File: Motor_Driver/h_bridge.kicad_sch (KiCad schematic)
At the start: 52 parts, among them M1 Motor_DC, M2 Motor_DC, Q10 PMOS, Q11 CSD18540Q5B, Q12 SQJ407EP, Q13 CSD18540Q5B, Q14 MMBT3904, Q3 CSD18540Q5B, Q4 CSD18540Q5B, Q5 SQJ407EP, Q6 PMOS, Q7 MMBT3904, Q8 MMBT3904, Q9 MMBT3904, U4 UCC27524D, U5 UCC27524D

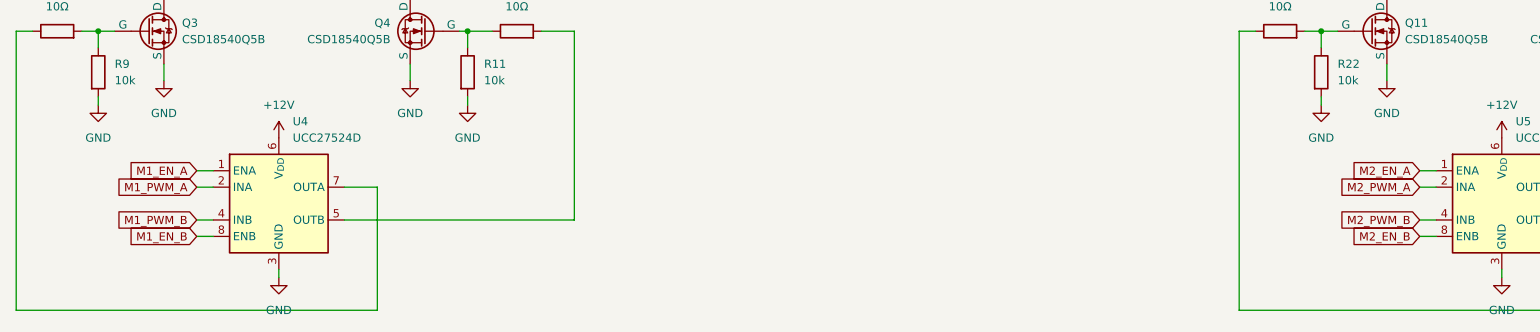
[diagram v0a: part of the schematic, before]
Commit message: Potential Finished Schematic Before Placements
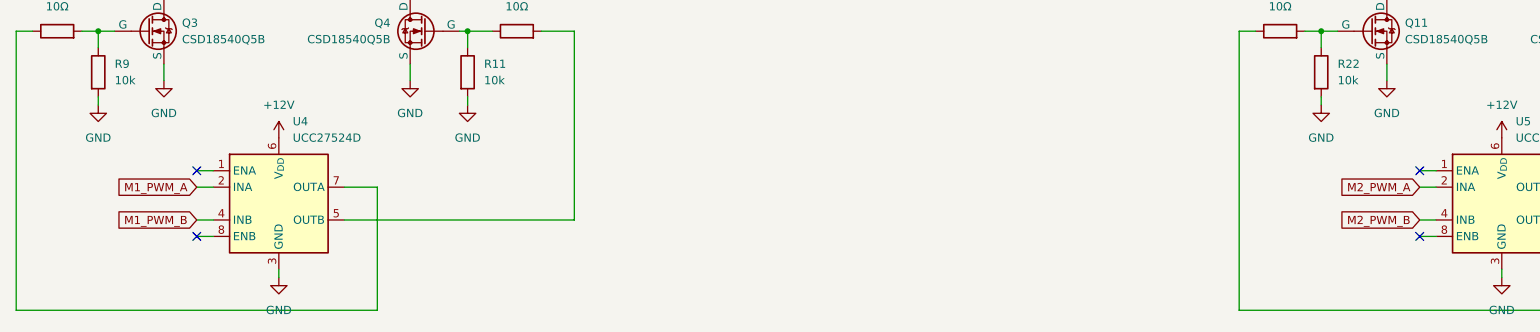
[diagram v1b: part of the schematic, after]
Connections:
- net M1_EN_A: no longer names the net of U4.1 (ENA)
- net M1_EN_B: no longer names the net of U4.8 (ENB)
- net M2_EN_A: no longer names the net of U5.1 (ENA)
- net M2_EN_B: no longer names the net of U5.8 (ENB)
- no-connect marks 0 -> 4
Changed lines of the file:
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@@
 		(color 0 0 0 0)
+	)
+	(no_connect
+		(at 292.1 190.5)
+	)
+	(no_connect
+		(at 102.87 190.5)
+	)
+	(no_connect
+		(at 292.1 180.34)
+	)
+	(no_connect
+		(at 102.87 180.34)
 	)
 	(wire
@@
 		)
 	)
-	(global_label "M2_EN_B"
-		(shape input)
-		(at 292.1 190.5 180)
-		(fields_autoplaced yes)
-		(effects
-			(font
-				(size 1.27 1.27)
-			)
-			(justify right)
-		)
-		(property "Intersheetrefs" "${INTERSHEET_REFS}"
-			(at 280.7692 190.5 0)
-			(hide yes)
-			(show_name no)
-			(do_not_autoplace no)
-			(effects
-				(font
-					(size 1.27 1.27)
-				)
-				(justify right)
-			)
-		)
-	)
-	(global_label "M1_EN_A"
-		(shape input)
-		(at 102.87 180.34 180)
-		(fields_autoplaced yes)
-		(effects
-			(font
-				(size 1.27 1.27)
-			)
-			(justify right)
-		)
-		(property "Intersheetrefs" "${INTERSHEET_REFS}"
-			(at 91.7206 180.34 0)
-			(hide yes)
-			(show_name no)
-			(do_not_autoplace no)
-			(effects
-				(font
-					(size 1.27 1.27)
-				)
-				(justify right)
-			)
-		)
-	)
 	(global_label "M1_PWM_A"
 		(shape input)
@@
 		)
 	)
-	(global_label "M2_EN_A"
-		(shape input)
-		(at 292.1 180.34 180)
-		(fields_autoplaced yes)
-		(effects
-			(font
-				(size 1.27 1.27)
-			)
-			(justify right)
-		)
-		(property "Intersheetrefs" "${INTERSHEET_REFS}"
-			(at 280.9506 180.34 0)
-			(hide yes)
-			(show_name no)
-			(do_not_autoplace no)
-			(effects
-				(font
-					(size 1.27 1.27)
-				)
-				(justify right)
-			)
-		)
-	)
 	(global_label "M1_P_A_ON"
 		(shape input)
@@
 			(hide yes)
 			(show_name no)
-			(do_not_autoplace no)
-			(effects
-				(font
-					(size 1.27 1.27)
-				)
-				(justify right)
-			)
-		)
-	)
-	(global_label "M1_EN_B"
-		(shape input)
-		(at 102.87 190.5 180)
-		(fields_autoplaced yes)
-		(effects
-			(font
-				(size 1.27 1.27)
-			)
-			(justify right)
-		)
-		(property "Intersheetrefs" "${INTERSHEET_REFS}"
-			(at 91.5392 190.5 0)
-			(hide yes)
-			(show_name no)
